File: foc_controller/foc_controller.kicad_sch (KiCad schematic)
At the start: 22 parts, among them J1 USB_B_Micro, U1 STM32G431KBUx, U2 AZ1117-3.3, Y1 16MHz

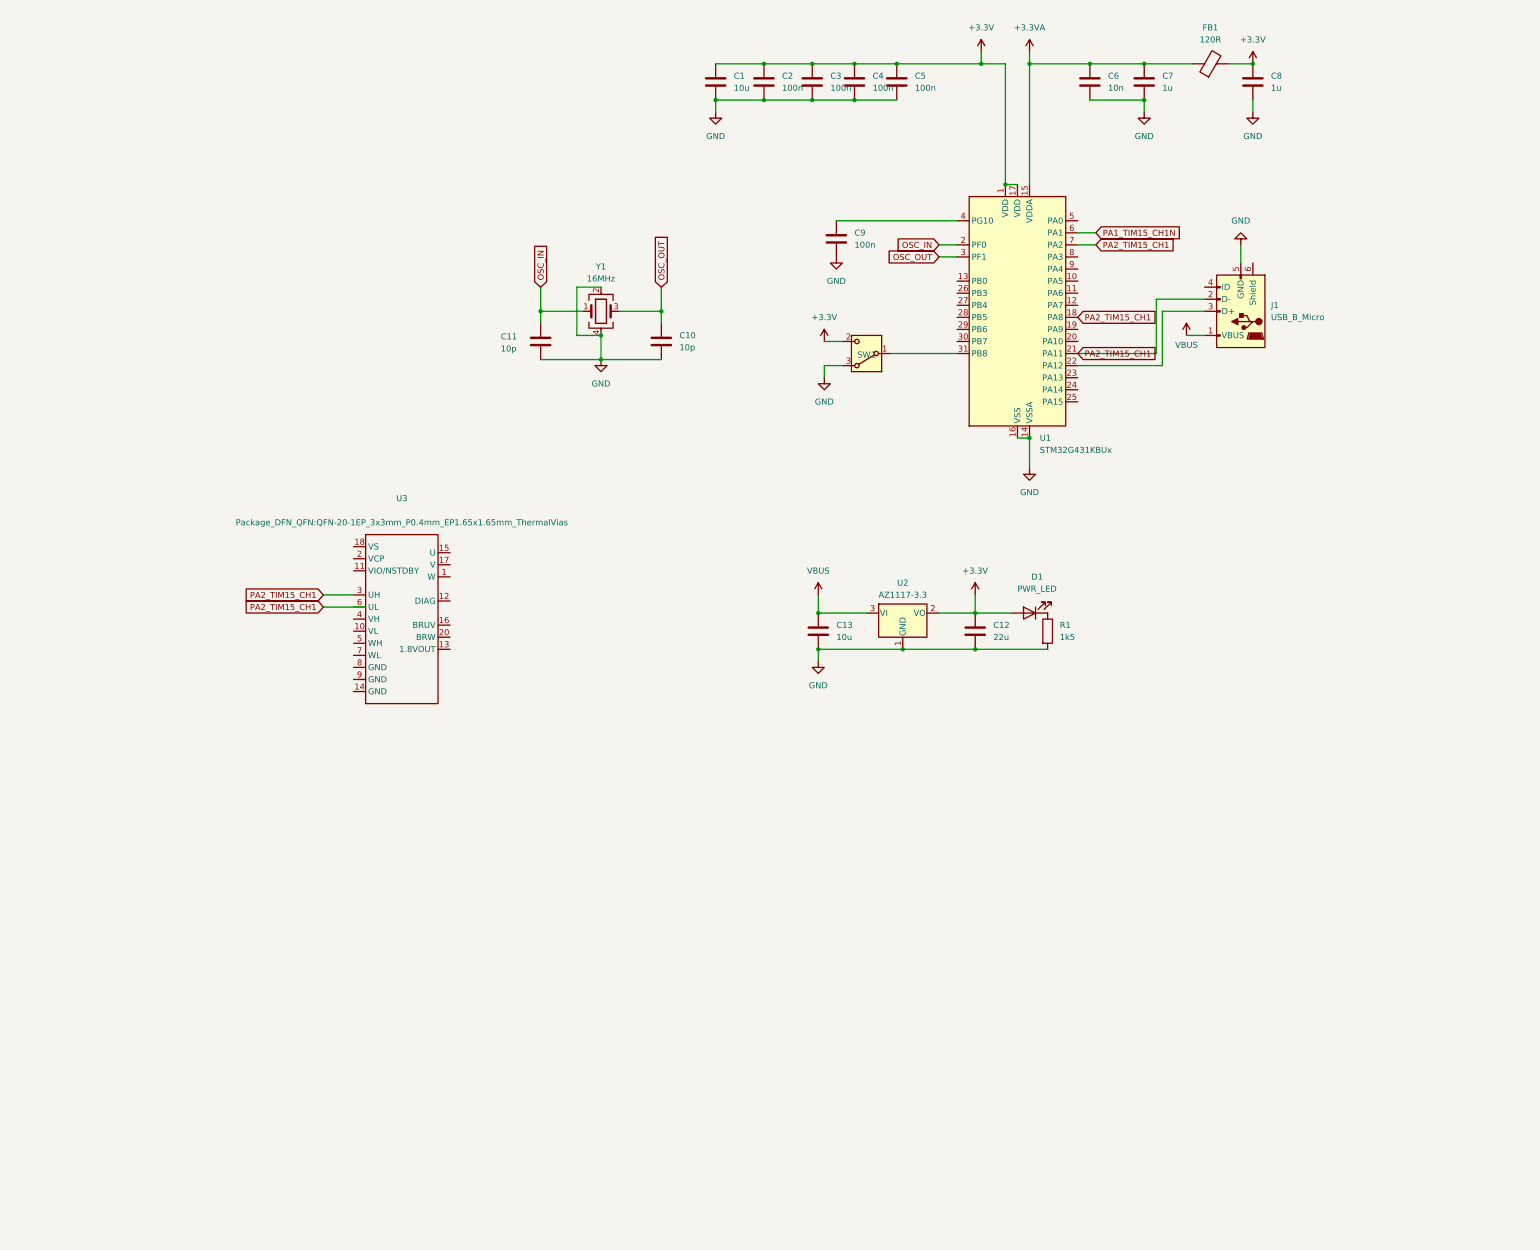
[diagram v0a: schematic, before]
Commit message: Pcb nearly complete
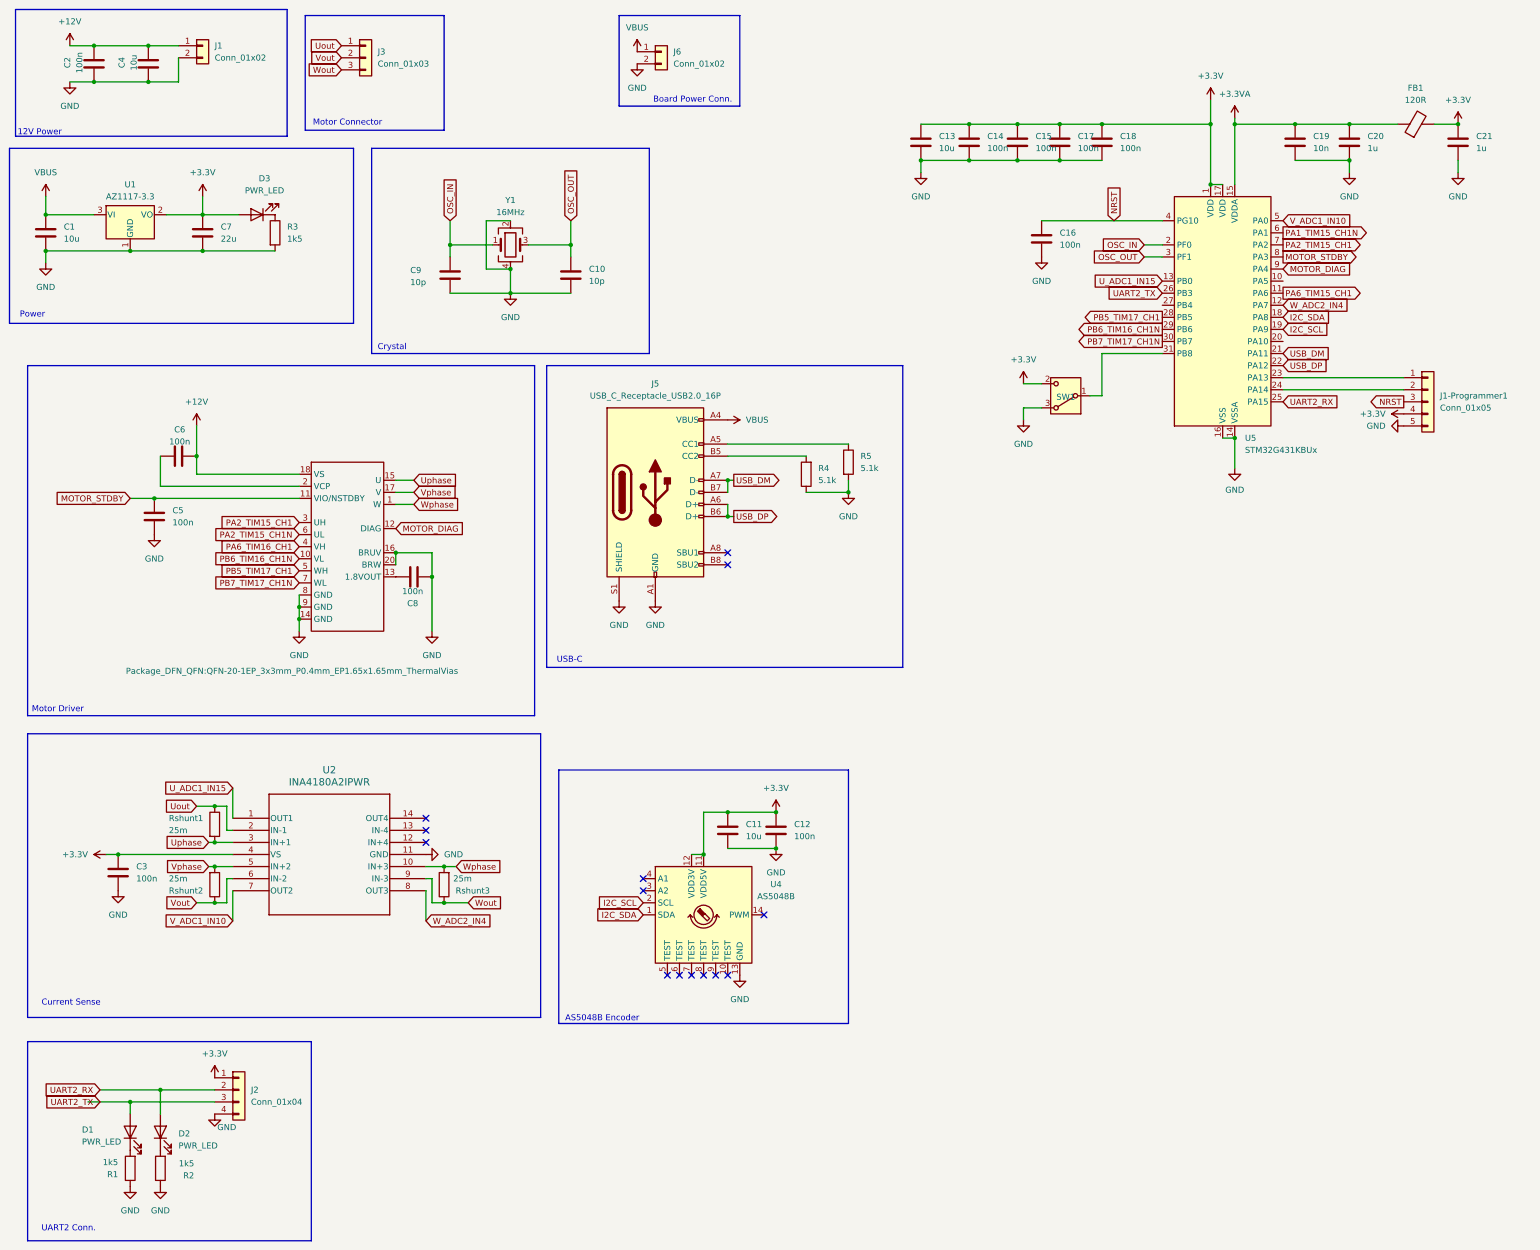
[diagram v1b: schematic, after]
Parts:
- removed J1: USB_B_Micro, symbol Connector:USB_B_Micro
- added C11, C4: 10u, Capacitor_SMD:C_0603_1608Metric, symbol Device:C
- added C12, C2, C3, C5, C6, C8: 100n, Capacitor_SMD:C_0603_1608Metric, symbol Device:C
- added D1, D2: PWR_LED, LED_SMD:LED_0603_1608Metric, symbol Device:LED
- added J1, J6: Conn_01x02, Connector_PinHeader_2.00mm:PinHeader_1x02_P2.00mm_Vertical, symbol Connector_Generic:Conn_01x02
- added J1-Programmer1: Conn_01x05, Connector_PinHeader_2.00mm:PinHeader_1x05_P2.00mm_Vertical, symbol Connector_Generic:Conn_01x05
- added J2: Conn_01x04, Connector_PinHeader_2.00mm:PinHeader_1x04_P2.00mm_Vertical, symbol Connector_Generic:Conn_01x04
- added J3: Conn_01x03, Connector_PinHeader_2.00mm:PinHeader_1x03_P2.00mm_Vertical, symbol Connector_Generic:Conn_01x03
- added J5: USB_C_Receptacle_USB2.0_16P, usb_connector_footprints:12402012E212A_AMP, symbol Connector:USB_C_Receptacle_USB2.0_16P
- added R1, R2: 1k5, Resistor_SMD:R_0603_1608Metric, symbol Device:R
- added R4, R5: 5.1k, Resistor_SMD:R_0603_1608Metric, symbol Device:R
- added Rshunt1, Rshunt2, Rshunt3: 25m, Resistor_SMD:R_0603_1608Metric, symbol Device:R
- added U2: INA4180A2IPWR, current_sense_footprints:PW14_TEX, symbol 2025-10-24_23-05-49:INA4180A2IPWR
- added U4: AS5048B, Package_SO:TSSOP-14_4.4x5mm_P0.65mm, symbol Sensor_Magnetic:AS5048B
- C1: renamed from C13; footprint (none) -> Capacitor_SMD:C_0603_1608Metric
- C10: footprint (none) -> Capacitor_SMD:C_0603_1608Metric
- C13: renamed from C1; footprint (none) -> Capacitor_SMD:C_0603_1608Metric
- C14: renamed from C2; footprint (none) -> Capacitor_SMD:C_0603_1608Metric
- C15: renamed from C3; footprint (none) -> Capacitor_SMD:C_0603_1608Metric
- C16: renamed from C9; footprint (none) -> Capacitor_SMD:C_0603_1608Metric
- C17: renamed from C4; footprint (none) -> Capacitor_SMD:C_0603_1608Metric
- C18: renamed from C5; footprint (none) -> Capacitor_SMD:C_0603_1608Metric
- C19: renamed from C6; footprint (none) -> Capacitor_SMD:C_0603_1608Metric
- C20: renamed from C7; footprint (none) -> Capacitor_SMD:C_0603_1608Metric
- C21: renamed from C8; footprint (none) -> Capacitor_SMD:C_0603_1608Metric
- C7: renamed from C12; footprint (none) -> Capacitor_SMD:C_0603_1608Metric
- C9: renamed from C11; footprint (none) -> Capacitor_SMD:C_0603_1608Metric
- D3: renamed from D1; footprint (none) -> LED_SMD:LED_0603_1608Metric
- FB1: footprint (none) -> Inductor_SMD:L_0603_1608Metric
- R3: renamed from R1; footprint (none) -> Resistor_SMD:R_0603_1608Metric
- SW1: footprint Button_Switch_THT:SW_Slide-03_Wuerth-WS-SLTV_10x2.5x6.4_P2.54mm -> button_footprint:SMT_FS
- U1: renamed from U2; footprint (none) -> voltage_regulator_footprints:SOT-223_DIO
- Y1: footprint (none) -> crystal_footprints:XTAL_ABM10AIG-16.000MHZ-4Z-T3
- renumbered U1 to U5
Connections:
- net +3.3V: now also C11.1, C12.1, C3.1, J1-Programmer1.4 (Pin_4), J2.1 (Pin_1), U2.4 (VS), U4.11 (VDD5V), U4.12 (VDD3V)
- net GND: now also U3.14 (GND), U3.16 (BRUV), U3.20 (BRW), U3.8 (GND), U3.9 (GND), C11.2, C12.2, C2.2, C3.2, C4.2, C5.2, C8.2, J1-Programmer1.5 (Pin_5), J1.2 (Pin_2), J2.4 (Pin_4), J5.A1 (GND), J5.A12 (GND), J5.B1 (GND), J5.B12 (GND), J5.S1 (SHIELD), J6.2 (Pin_2), R1.1, R2.1, R4.1, R5.2, U2.11 (GND), U4.13 (GND)
- net PA2_TIM15_CH1: no longer U5.18 (PA8), U5.21 (PA11)
- net VBUS: now also J5.A4 (VBUS), J5.A9 (VBUS), J5.B4 (VBUS), J5.B9 (VBUS), J6.1 (Pin_1)
- net NRST: now reaches C16.1, U5.4 (PG10)
- net NRST: now also J1-Programmer1.3 (Pin_3)
- net Wphase: now reaches U3.1 (W)
- net Wphase: now also Rshunt3.2, U2.10 (IN+3)
- net PB6_TIM16_CH1N: now reaches U3.10 (VL)
- net PB6_TIM16_CH1N: now also U5.29 (PB6)
- net MOTOR_STDBY: now reaches U3.11 (VIO/NSTDBY)
- net MOTOR_STDBY: now also U5.8 (PA3), C5.1
- net MOTOR_DIAG: now reaches U3.12 (DIAG)
- net MOTOR_DIAG: now also U5.9 (PA4)
- net at U3.13 (1.8VOUT): now also C8.1
- net Uphase: now reaches U3.15 (U)
- net Uphase: now also Rshunt1.2, U2.3 (IN+1)
- net Vphase: now reaches U3.17 (V)
- net Vphase: now also Rshunt2.2, U2.5 (IN+2)
- net +12V: now reaches U3.18 (VS)
- net +12V: now also C2.1, C4.1, C6.1, J1.1 (Pin_1)
- net at U3.2 (VCP): now also C6.2
- net PA6_TIM16_CH1: now reaches U3.4 (VH)
- net PB5_TIM17_CH1: now reaches U3.5 (WH)
- net PB5_TIM17_CH1: now also U5.28 (PB5)
- net PA2_TIM15_CH1N: now reaches U3.6 (UL)
- net PB7_TIM17_CH1N: now reaches U3.7 (WL)
- net PB7_TIM17_CH1N: now also U5.30 (PB7)
- net USB_DP: now reaches U5.22 (PA12)
- net USB_DP: now also J5.A6 (D+), J5.B6 (D+)
- net PA6_TIM15_CH1: now reaches U5.11 (PA6)
- net W_ADC2_IN4: now reaches U5.12 (PA7)
- net W_ADC2_IN4: now also U2.8 (OUT3)
- net U_ADC1_IN15: now reaches U5.13 (PB0)
- net U_ADC1_IN15: now also U2.1 (OUT1)
- net I2C_SCL: now reaches U5.19 (PA9)
- net I2C_SCL: now also U4.2 (SCL)
- net at U5.23 (PA13): now also J1-Programmer1.1 (Pin_1)
- net at U5.24 (PA14): now also J1-Programmer1.2 (Pin_2)
- net UART2_RX: now reaches U5.25 (PA15)
- net UART2_RX: now also D2.2 (A), J2.2 (Pin_2)
- net UART2_TX: now reaches U5.26 (PB3)
- net UART2_TX: now also D1.2 (A), J2.3 (Pin_3)
- net V_ADC1_IN10: now reaches U5.5 (PA0)
- net V_ADC1_IN10: now also U2.7 (OUT2)
- new net: J5.B5 (CC2), R4.2
- new net: D1.1 (K), R1.2
- new net: J5.A5 (CC1), R5.1
- new net: D2.1 (K), R2.2
- new net I2C_SDA: U4.1 (SDA), U5.18 (PA8)
- new net USB_DM: J5.A7 (D-), J5.B7 (D-), U5.21 (PA11)
- new net Uout: J3.1 (Pin_1), Rshunt1.1, U2.2 (IN-1)
- new net Vout: J3.2 (Pin_2), Rshunt2.1, U2.6 (IN-2)
- new net Wout: J3.3 (Pin_3), Rshunt3.1, U2.9 (IN-3)
- no-connect marks 0 -> 14
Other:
- note added: "12V Power"
- note added: "AS5048B Encoder"
- note added: "Board Power Conn."
- note added: "Crystal"
- note added: "Current Sense"
- note added: "Motor Connector"
- note added: "Motor Driver"
- note added: "Power"
- note added: "UART2 Conn."
- note added: "USB-C"
- moved on the sheet: C1, C10, C13, C14, C15, C16, C17, C18, C19, C20, C21, C7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
